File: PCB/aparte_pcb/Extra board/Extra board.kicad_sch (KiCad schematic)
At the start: 4 parts, among them J1 Conn_01x10_Pin, J2 Conn_01x04_Pin, J3 Conn_01x10_Socket, U1 MCP23008-xP

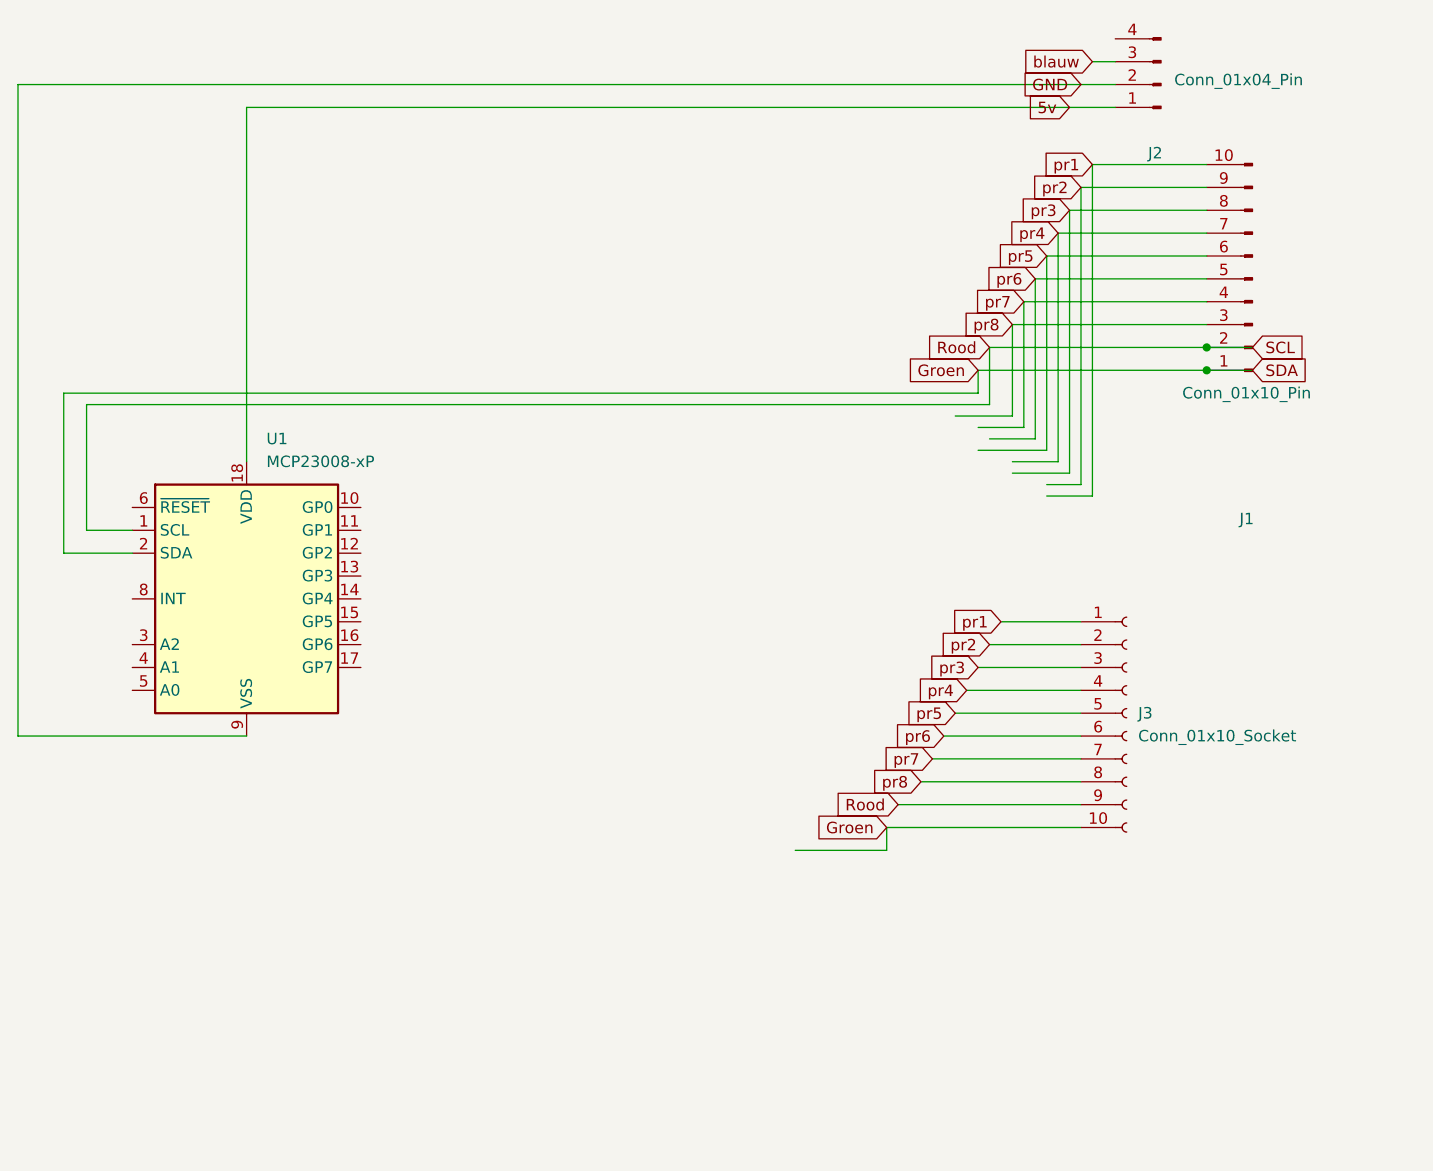
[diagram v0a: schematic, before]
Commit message: extra PCB changes
Multi-line description of commit,
feel free to be detailed.

Signed-off-by: Abel Tim <git@abeltim.com>
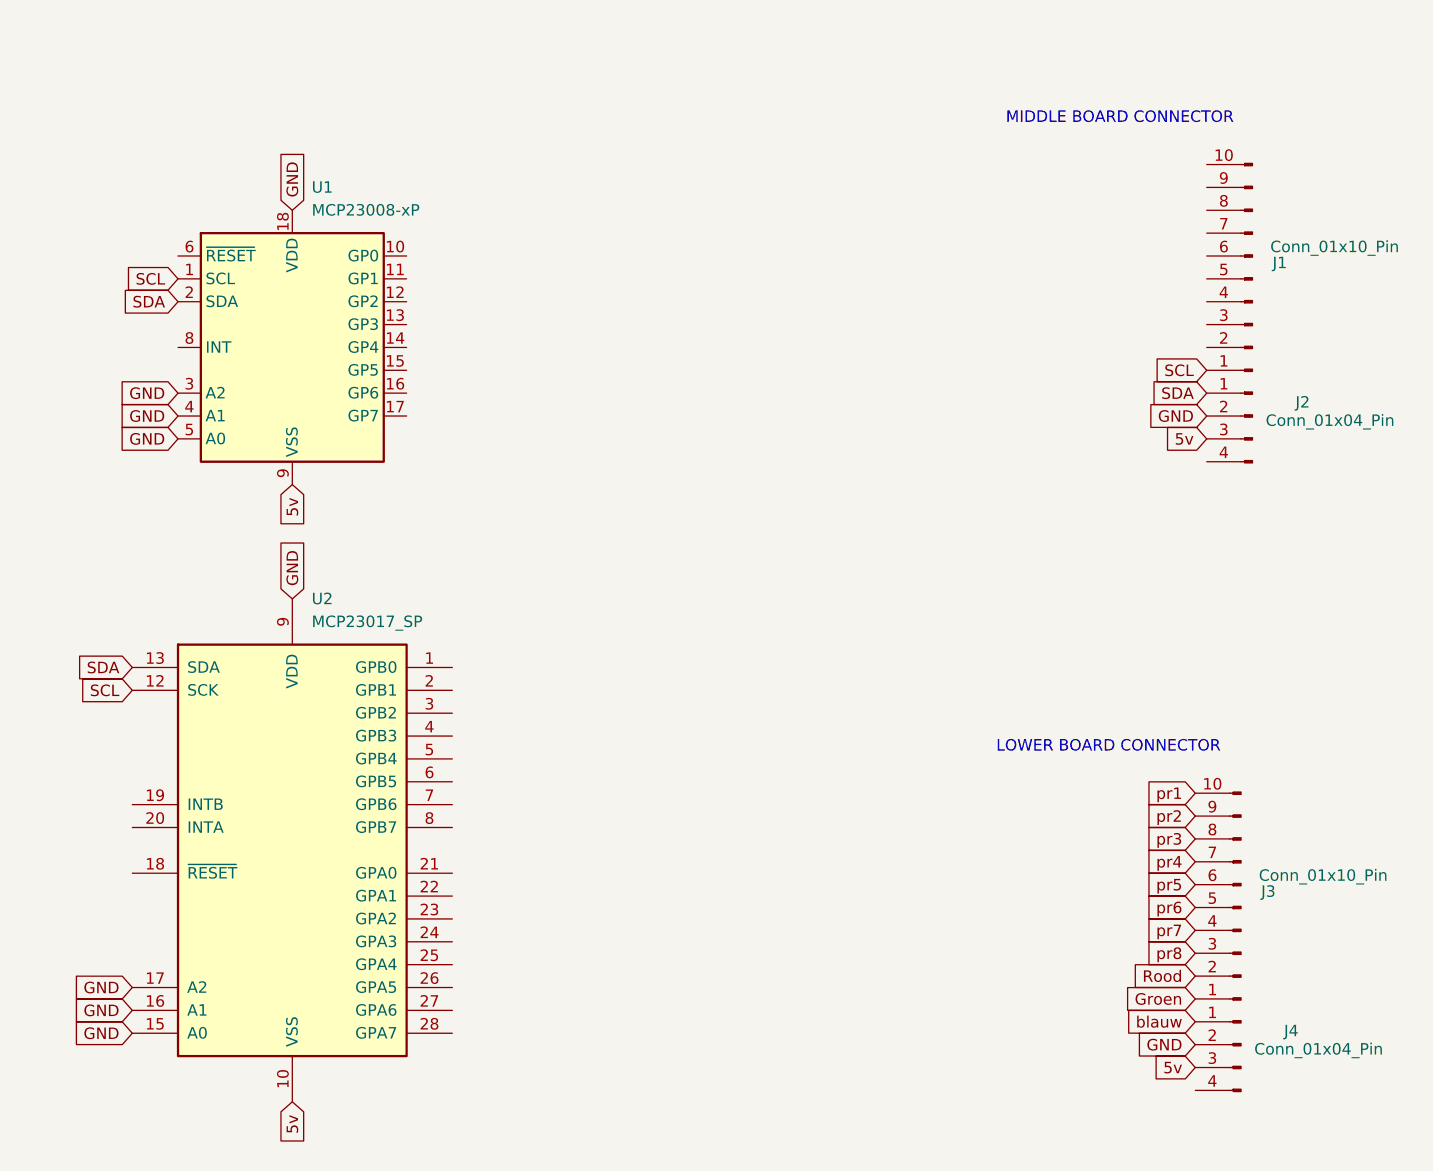
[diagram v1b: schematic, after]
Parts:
- removed J3: Conn_01x10_Socket, symbol Connector:Conn_01x10_Socket
- added J3: Conn_01x10_Pin, symbol Connector:Conn_01x10_Pin
- added J4: Conn_01x04_Pin, symbol Connector:Conn_01x04_Pin
- added U2: MCP23017_SP, Package_DIP:DIP-28_W7.62mm, symbol Interface_Expansion:MCP23017_SP
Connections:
- net 5v: now also J2.3 (Pin_3), U1.9 (VSS), J4.3 (Pin_3), U2.10 (VSS); no longer J2.1 (Pin_1), U1.18 (VDD)
- net GND: now also U1.18 (VDD), U1.3 (A2), U1.4 (A1), U1.5 (A0), J4.2 (Pin_2), U2.15 (A0), U2.16 (A1), U2.17 (A2), U2.9 (VDD); no longer U1.9 (VSS)
- net Groen: now also J3.1 (Pin_1); no longer J1.1 (Pin_1), U1.2 (SDA)
- net Rood: now also J3.2 (Pin_2); no longer J1.2 (Pin_2), U1.1 (SCL)
- net blauw: now also J4.1 (Pin_1); no longer J2.3 (Pin_3)
- net pr1: now also J3.10 (Pin_10); no longer J1.10 (Pin_10)
- net pr2: now also J3.9 (Pin_9); no longer J1.9 (Pin_9)
- net pr3: now also J3.8 (Pin_8); no longer J1.8 (Pin_8)
- net pr4: now also J3.7 (Pin_7); no longer J1.7 (Pin_7)
- net pr5: now also J3.6 (Pin_6); no longer J1.6 (Pin_6)
- net pr6: now also J3.5 (Pin_5); no longer J1.5 (Pin_5)
- net pr7: now also J3.4 (Pin_4); no longer J1.4 (Pin_4)
- net pr8: now also J3.3 (Pin_3); no longer J1.3 (Pin_3)
- new net SCL: J1.1 (Pin_1), U1.1 (SCL), U2.12 (SCK)
- new net SDA: J2.1 (Pin_1), U1.2 (SDA), U2.13 (SDA)
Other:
- note added: "LOWER BOARD CONNECTOR"
- note added: "MIDDLE BOARD CONNECTOR"
- moved on the sheet: J2
